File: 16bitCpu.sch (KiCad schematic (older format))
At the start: 0 parts

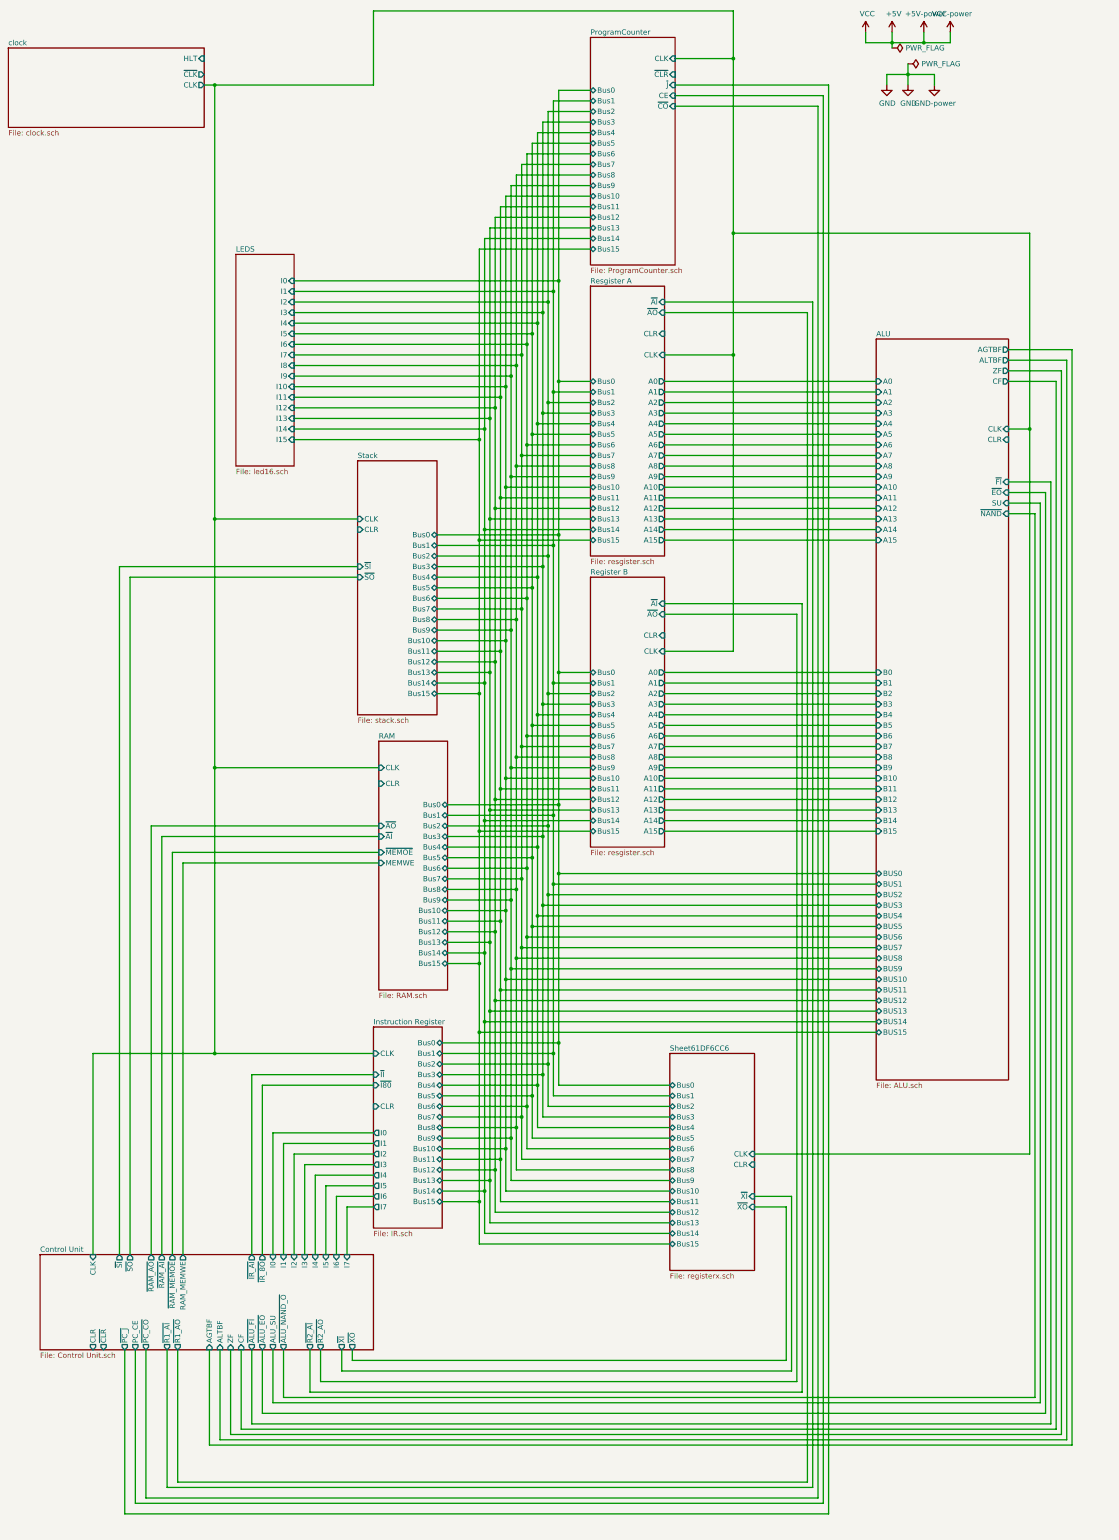
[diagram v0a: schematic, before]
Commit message: fixed almost all errors
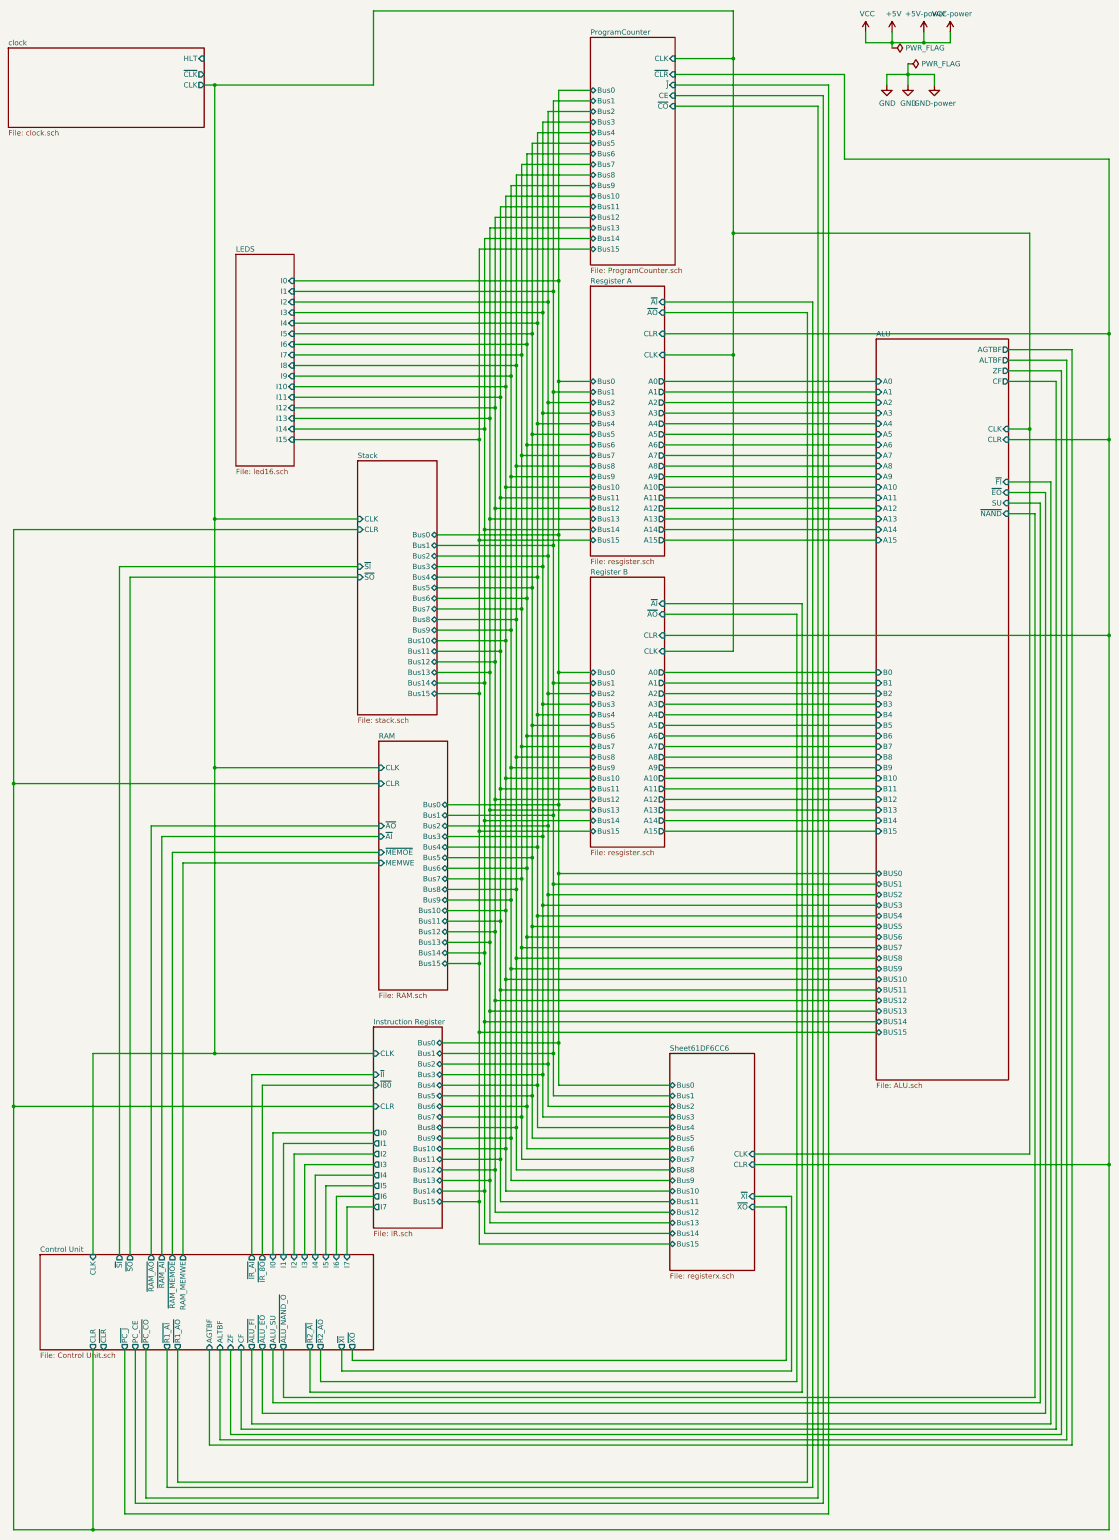
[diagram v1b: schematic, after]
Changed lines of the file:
@@
 Wire Wire Line
 	7450 2650 10250 2650
-Wire Wire Line
-	10250 2650 10250 4500
 Connection ~ 7450 2650
 Wire Wire Line
@@
 Wire Wire Line
 	2500 14100 2500 13200
+Wire Wire Line
+	1400 13200 1400 14900
+Wire Wire Line
+	1400 14900 11000 14900
+Wire Wire Line
+	11000 4600 10050 4600
+Wire Wire Line
+	11000 1950 8500 1950
+Wire Wire Line
+	8500 1950 8500 1150
+Wire Wire Line
+	8500 1150 6900 1150
+Connection ~ 11000 4600
+Wire Wire Line
+	6800 6450 11000 6450
+Connection ~ 11000 6450
+Wire Wire Line
+	11000 6450 11000 4600
+Wire Wire Line
+	7650 11450 11000 11450
+Wire Wire Line
+	11000 6450 11000 11450
+Connection ~ 11000 11450
+Wire Wire Line
+	11000 11450 11000 14900
+Wire Wire Line
+	10250 2650 10250 4500
+Wire Wire Line
+	6800 3600 11000 3600
+Wire Wire Line
+	11000 1950 11000 3600
+Connection ~ 11000 3600
+Wire Wire Line
+	11000 3600 11000 4600
+Wire Wire Line
+	1400 14900 650  14900
+Wire Wire Line
+	650  5450 3900 5450
+Connection ~ 1400 14900
+Wire Wire Line
+	4100 7850 650  7850
+Connection ~ 650  7850
+Wire Wire Line
+	650  7850 650  5450
+Wire Wire Line
+	4050 10900 650  10900
+Wire Wire Line
+	650  7850 650  10900
+Connection ~ 650  10900
+Wire Wire Line
+	650  10900 650  14900
 $EndSCHEMATC
